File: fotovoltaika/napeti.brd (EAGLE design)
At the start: 25.1 x 39.4 mm, 6 parts

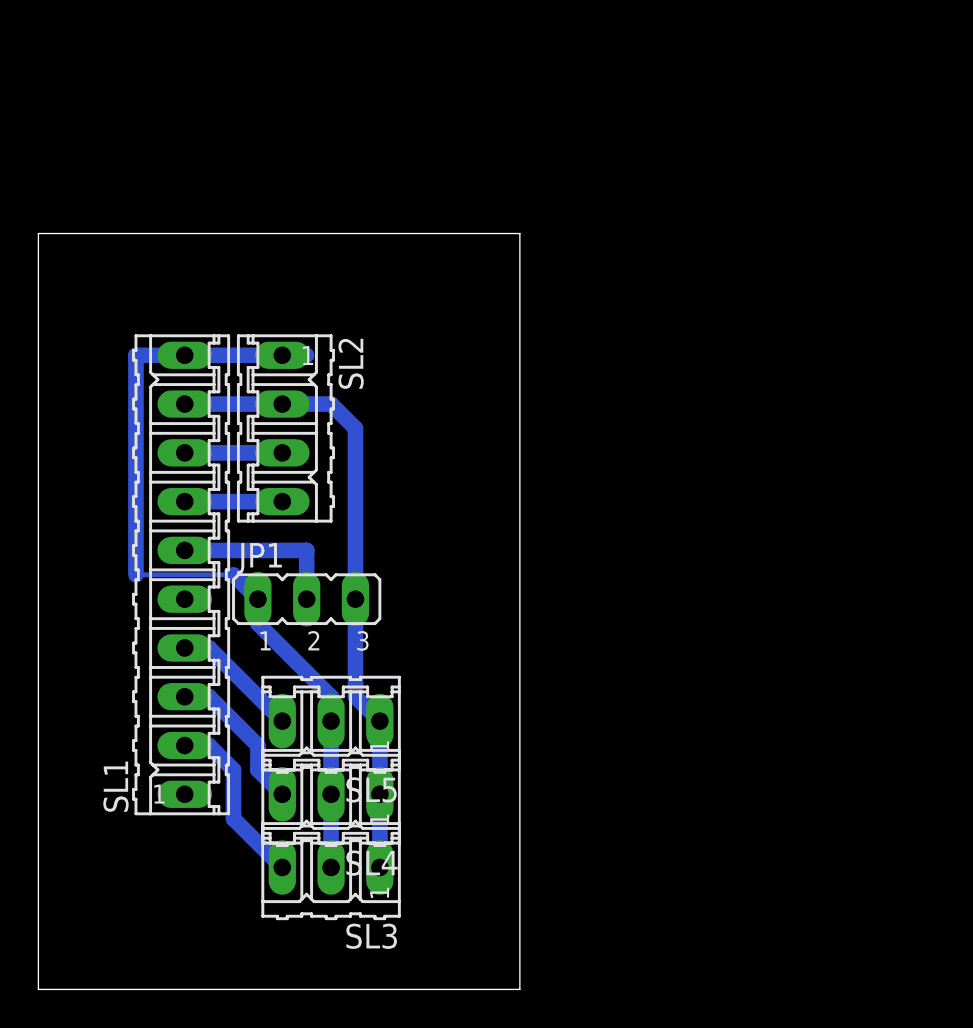
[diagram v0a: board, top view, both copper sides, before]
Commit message: upravy desek
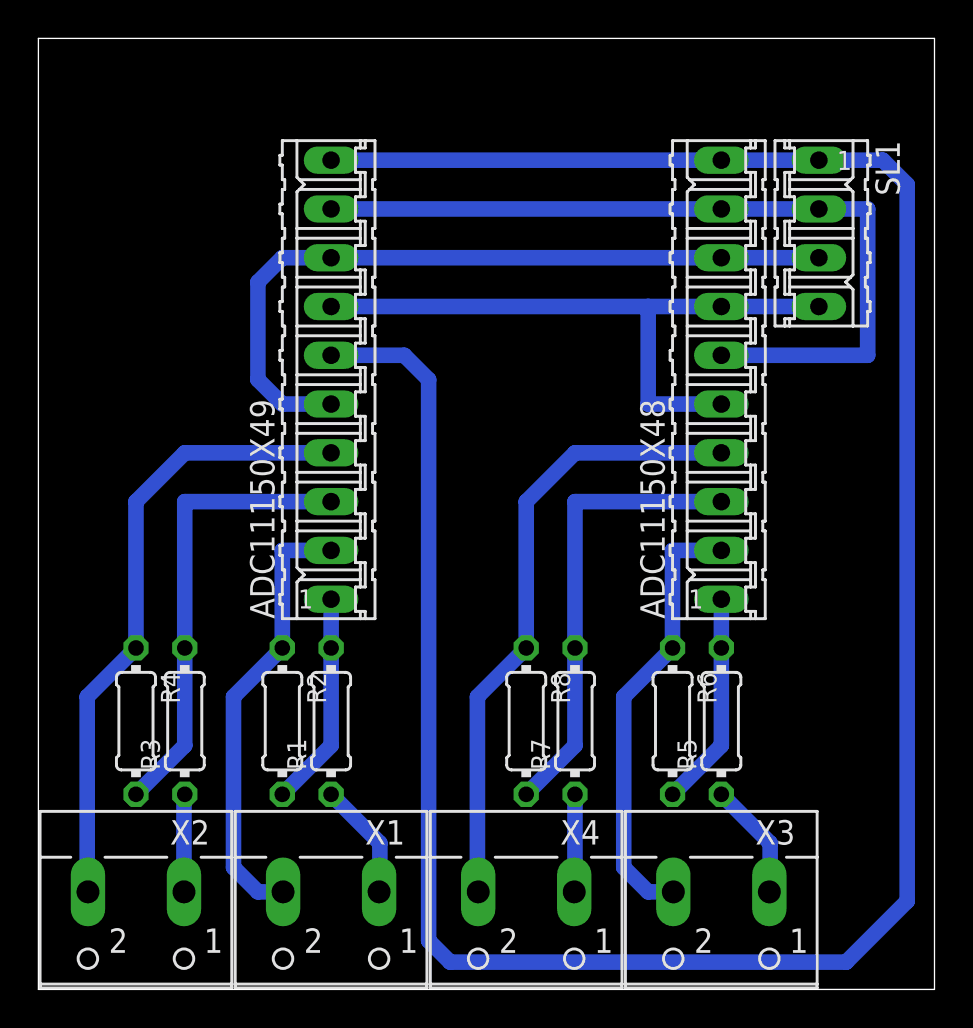
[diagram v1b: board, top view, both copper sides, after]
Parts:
- removed JP1: (no value), jumper:JP2
- removed SL2: (no value), con-amp-quick:04P
- removed SL3, SL4, SL5: (no value), con-amp-quick:03P
- added ADC11150X48, ADC11150X49: (no value), con-amp-quick:10P
- added R1, R3, R5: 10k, rcl:0204/7
- added R2: 2k7, rcl:0204/7
- added R4, R6: 4k7, rcl:0204/7
- added R7, R8: (no value), rcl:0204/7
- added X1, X2, X3, X4: (no value), con-wago-500:W237-102
- SL1: device con-amp-quick:10P -> con-amp-quick:04P
- moved SL1 37.5 mm to (40.6, 39.4), turned to 270 degrees
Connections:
- removed net +5V: JP1.1, SL1.10, SL2.1, SL3.2, SL4.2, SL5.2
- removed net N$11: SL1.7, SL2.4
- new net 5V: ADC11150X48.10, ADC11150X49.10, ADC11150X49.6, SL1.1
- new net N$1: ADC11150X48.1, R5.2, R6.2
- new net N$10: ADC11150X49.2, R2.1, X1.2
- new net N$13: ADC11150X49.3, R3.2, R4.2
- new net N$3: ADC11150X48.2, R6.1, X3.2
- new net N$4: ADC11150X48.3, R7.2, R8.2
- new net N$8: R7.1, X4.1
- new net N$9: ADC11150X49.1, R1.2, R2.2
- new net SCL: ADC11150X48.5, ADC11150X48.7, ADC11150X49.7, SL1.4
- new net SDA: ADC11150X48.8, ADC11150X49.5, ADC11150X49.8, SL1.3
- net GND: now also ADC11150X48.6, ADC11150X48.9, ADC11150X49.9, SL1.2; no longer JP1.3, SL1.9, SL2.2, SL3.1, SL4.1, SL5.1
- net N$14: now also ADC11150X49.4, R4.1, X2.2; no longer JP1.2, SL1.6
- net N$2: now also R1.1, X1.1; no longer SL1.8, SL2.3
- net N$5: now also R3.1, X2.1; no longer SL1.2, SL3.3
- net N$6: now also ADC11150X48.4, R8.1, X4.2; no longer SL1.3, SL4.3
- net N$7: now also R5.1, X3.1; no longer SL1.4, SL5.3
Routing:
- net 5V: track 0.00 -> 129.3 mm
- net +5V: track 42.7 -> 0.00 mm
- net SDA: track 0.00 -> 39.2 mm
- net SCL: track 0.00 -> 34.3 mm
- net N$6: track 7.93 -> 32.6 mm
- net N$4: track 0.00 -> 23.9 mm
- net N$13: track 0.00 -> 23.9 mm
- net N$14: track 8.89 -> 32.6 mm
- net N$3: track 0.00 -> 23.2 mm
- net N$10: track 0.00 -> 23.2 mm
- net N$9: track 0.00 -> 11.2 mm
- net N$1: track 0.00 -> 11.2 mm
- net GND: track 32.8 -> 43.2 mm
- net N$8: track 0.00 -> 5.10 mm
- net N$11: track 5.08 -> 0.00 mm
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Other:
- board size 25.1 x 39.4 mm -> 46.7 x 49.5 mm
